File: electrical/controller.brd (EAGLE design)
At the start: 101.6 x 25.4 mm, 29 parts, among them Q1 IRLIB9343PBF-ND, U1 MCP6002, U2 POLOLU_U1V11F5, U3 MCP4725, U4 MCP4725

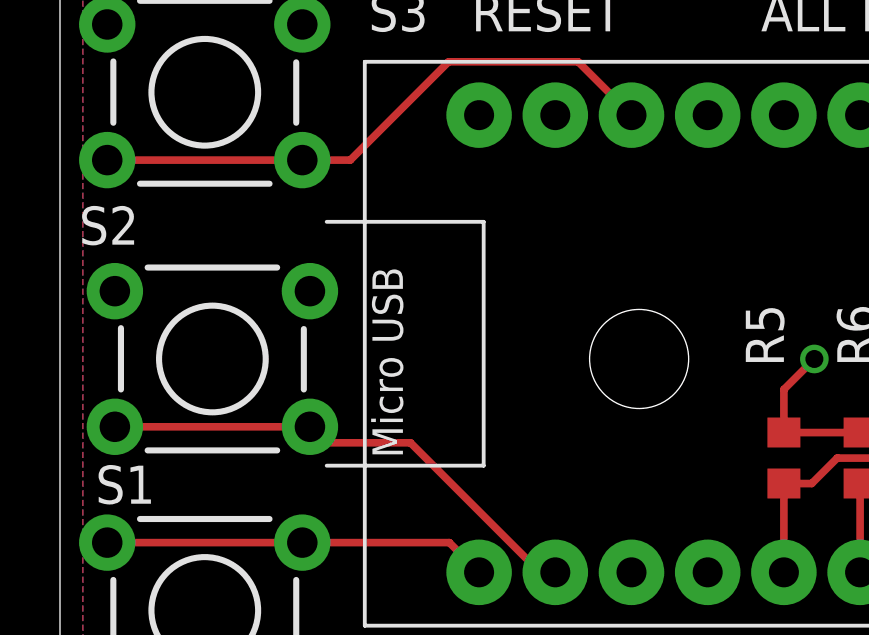
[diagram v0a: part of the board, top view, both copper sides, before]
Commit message: Small board fixes
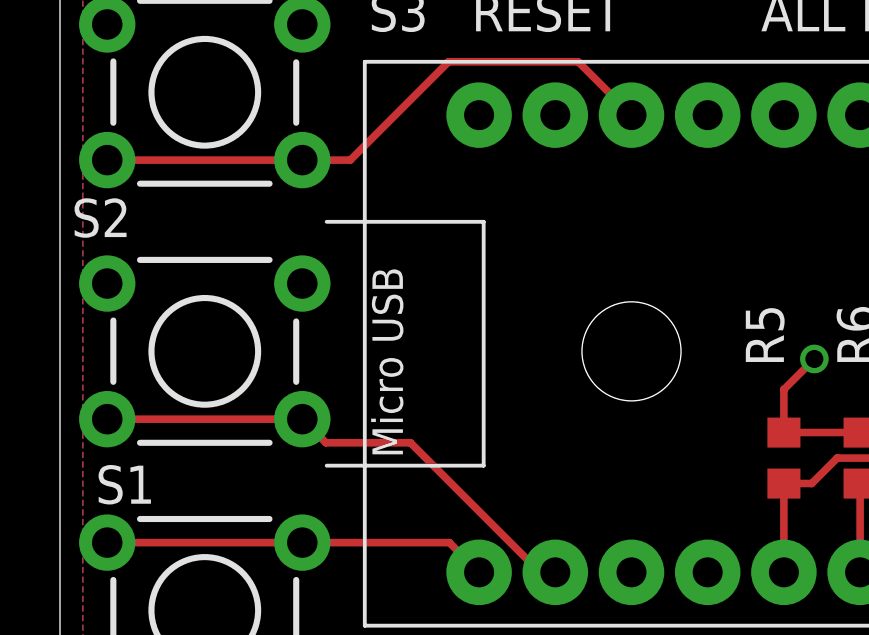
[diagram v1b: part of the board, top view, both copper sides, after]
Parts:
- moved S2 0.36 mm to (4.83, 12.7)
- moved U$8 0.36 mm to (19.1, 12.7)
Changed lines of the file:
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@@
 <attribute name="NAME" x="3.175" y="8.89" size="1.27" layer="25" font="vector" ratio="10" rot="R180"/>
 </element>
-<element name="S2" library="pie" package="TACTILE-PTH" value="" x="5.08" y="12.446">
-<attribute name="PIE-INT-REF-NUM" value="pth_pushbutton" x="5.08" y="12.446" size="1.778" layer="27" display="off"/>
+<element name="S2" library="pie" package="TACTILE-PTH" value="" x="4.826" y="12.7">
+<attribute name="PIE-INT-REF-NUM" value="pth_pushbutton" x="4.826" y="12.7" size="1.778" layer="27" display="off"/>
 </element>
 <element name="C1" library="SparkFun-Capacitors" package="CPOL-RADIAL-1000UF-63V" value="10mF" x="96.012" y="20.066" smashed="yes">
@@
 <attribute name="VALUE" x="74.803" y="24.13" size="1.27" layer="27" font="vector" rot="R270"/>
 </element>
-<element name="U$8" library="pie" package="STAND-OFF-TIGHT" value="" x="19.304" y="12.446"/>
+<element name="U$8" library="pie" package="STAND-OFF-TIGHT" value="" x="19.05" y="12.7"/>
 <element name="U$12" library="pie" package="STAND-OFF-TIGHT" value="" x="70.358" y="12.7"/>
 </elements>
@@
 <wire x1="16.002" y1="5.334" x2="11.684" y2="9.652" width="0.254" layer="1"/>
 <wire x1="11.684" y1="9.652" x2="8.8646" y2="9.652" width="0.254" layer="1"/>
-<wire x1="8.8646" y1="9.652" x2="8.3312" y2="10.1854" width="0.254" layer="1"/>
-<wire x1="8.3312" y1="10.1854" x2="1.8288" y2="10.1854" width="0.254" layer="1"/>
+<wire x1="8.8646" y1="9.652" x2="8.0772" y2="10.4394" width="0.254" layer="1"/>
+<wire x1="8.0772" y1="10.4394" x2="1.5748" y2="10.4394" width="0.254" layer="1"/>
 </signal>
 <signal name="VBAT">
